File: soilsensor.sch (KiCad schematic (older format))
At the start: 5 parts, among them J1 CONN_01X07, U1 DS18B20U, U2 RFD77101

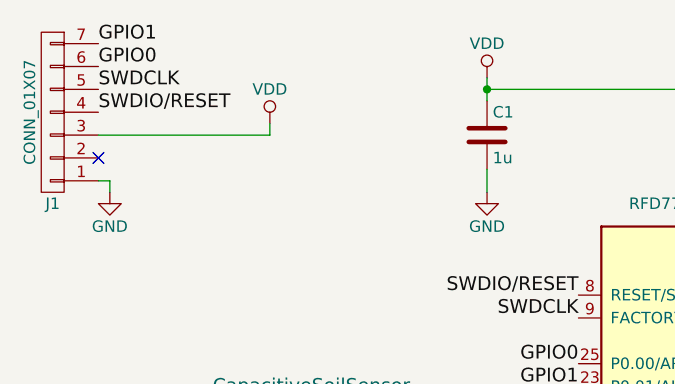
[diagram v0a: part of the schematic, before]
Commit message: update schematics
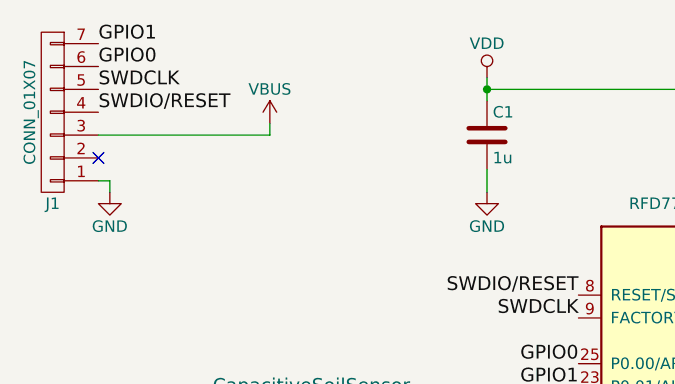
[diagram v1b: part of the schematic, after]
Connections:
- net VDD: no longer J1.3 (P3)
- new net VBUS: J1.3 (P3)
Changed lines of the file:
@@
 Connection ~ 5300 1600
-$Comp
-L VDD #PWR04
-U 1 1 5956777F
-P 4350 1750
-F 0 "#PWR04" H 4350 1600 50  0001 C CNN
-F 1 "VDD" H 4350 1900 50  0000 C CNN
-F 2 "" H 4350 1750 50  0001 C CNN
-F 3 "" H 4350 1750 50  0001 C CNN
-	1    4350 1750
-	1    0    0    -1
-$EndComp
 $Comp
 L GND #PWR05
@@
 	3650 3650 3950 3650
 Connection ~ 3950 4400
+$Comp
+L VBUS #PWR?
+U 1 1 59F88CC6
+P 4350 1750
+F 0 "#PWR?" H 4350 1600 50  0001 C CNN
+F 1 "VBUS" H 4350 1900 50  0000 C CNN
+F 2 "" H 4350 1750 50  0001 C CNN
+F 3 "" H 4350 1750 50  0001 C CNN
+	1    4350 1750
+	1    0    0    -1
+$EndComp
 $EndSCHEMATC
